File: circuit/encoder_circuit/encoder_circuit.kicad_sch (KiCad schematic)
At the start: 6 parts, among them J1 Conn_01x04

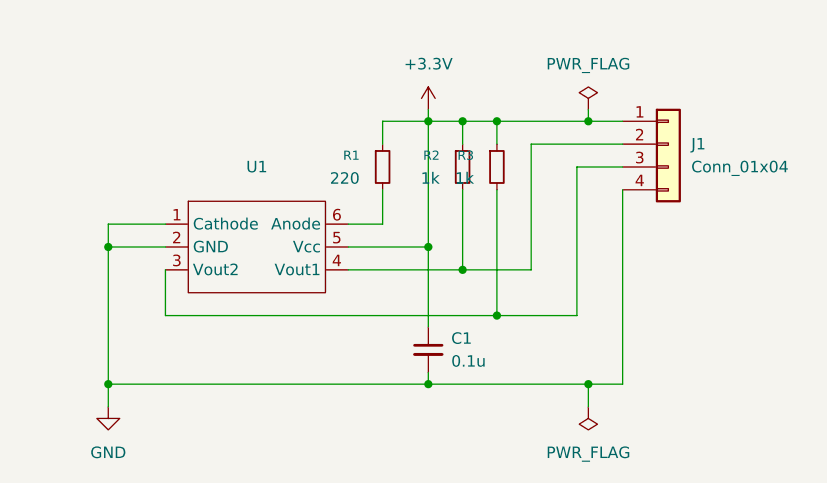
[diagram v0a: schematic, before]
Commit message: 整理
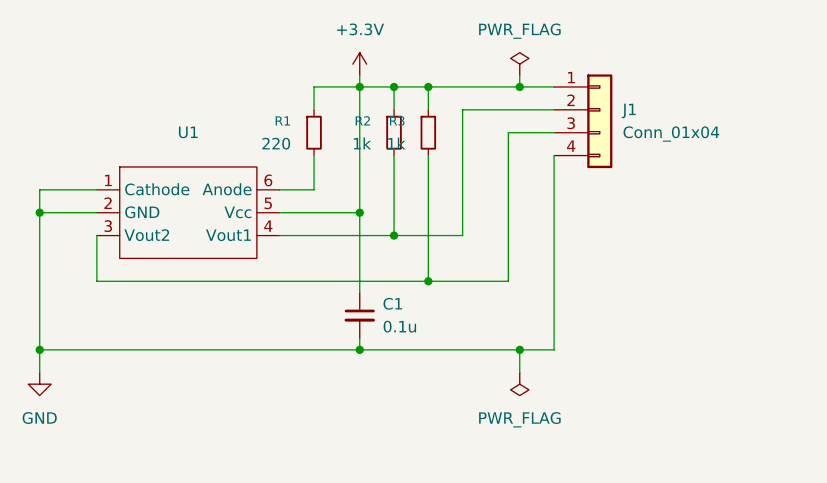
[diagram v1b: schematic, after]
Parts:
- U1: footprint mylib:NJL5820R -> OptoDevice:NJL5820R
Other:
- moved on the sheet: C1, J1, R1, R2, R3, U1
